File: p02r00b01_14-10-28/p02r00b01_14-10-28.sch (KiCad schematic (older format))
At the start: 0 parts

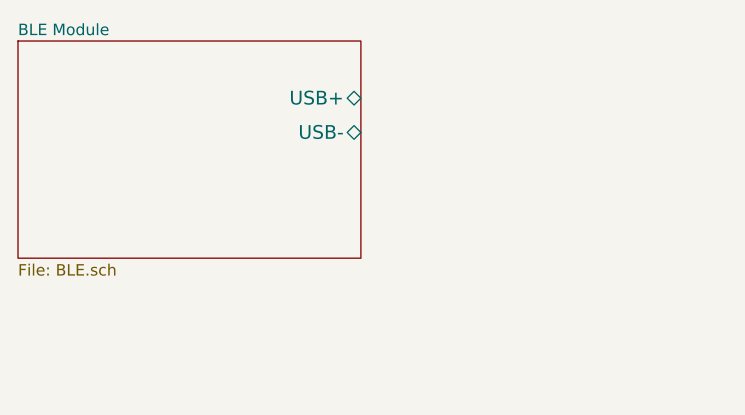
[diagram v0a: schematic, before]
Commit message: adding more files. Still dont know what am i doing.
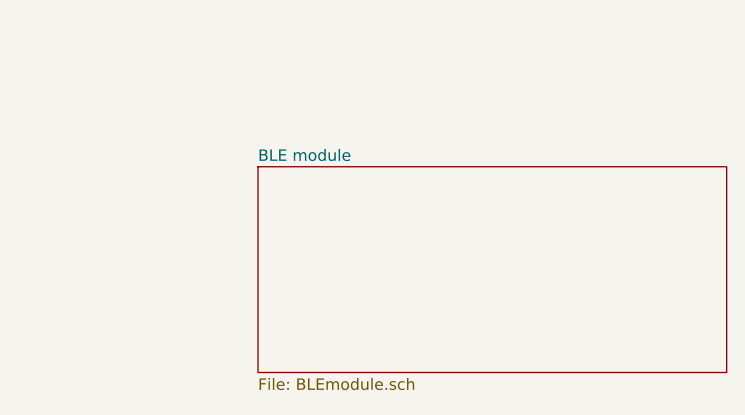
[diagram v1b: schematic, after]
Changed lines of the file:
@@
 LIBS:contrib
 LIBS:valves
+LIBS:p02r00b01_14-10-28-cache
 LIBS:proximity-cache
 EELAYER 27 0
@@
 Sheet 1 2
 Title ""
-Date "28 oct 2014"
+Date "31 oct 2014"
 Rev ""
 Comp ""
@@
 $EndDescr
 $Sheet
-S 1500 1450 1500 950
-U 544F4556
-F0 "BLE Module" 50
-F1 "BLE.sch" 50
-F2 "USB+" B R 3000 1700 60
-F3 "USB-" B R 3000 1850 60
+S 2550 2000 2050 900
+U 545385E5
+F0 "BLE module" 50
+F1 "BLEmodule.sch" 50
 $EndSheet
 $EndSCHEMATC
